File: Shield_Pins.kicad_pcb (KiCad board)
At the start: 2 copper layers, 76 x 38.3 mm, 19 parts, among them J1 Conn_01x04_Male, J2 Conn_01x06_Male, J3 Conn_01x06_Male, J4 Conn_01x04_Male, J5 Conn_01x01_Male, J6 Conn_01x06_Male, J7 Conn_01x15_Male, J8 Conn_01x15_Male, J9 Conn_01x02_Male, U1 ADXL343, U2 AZ1117

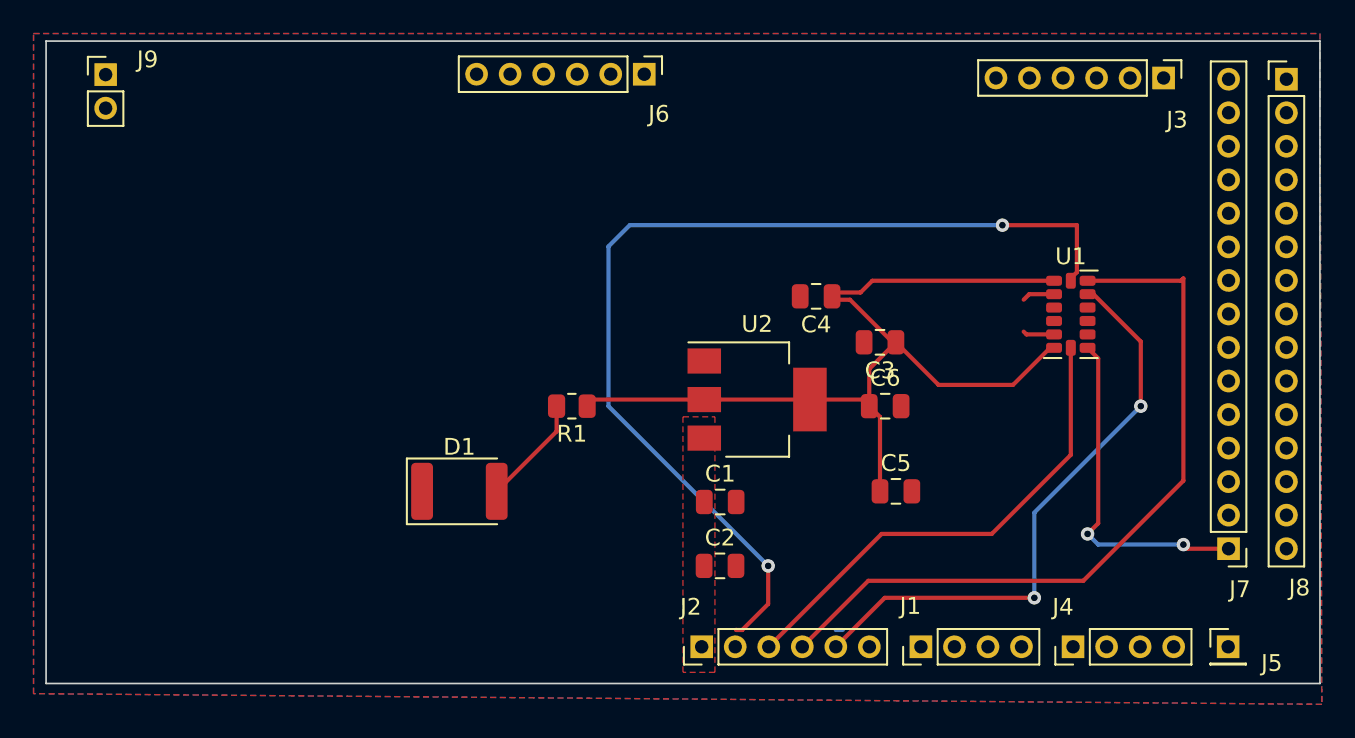
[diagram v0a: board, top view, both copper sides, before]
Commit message: Finished shield design
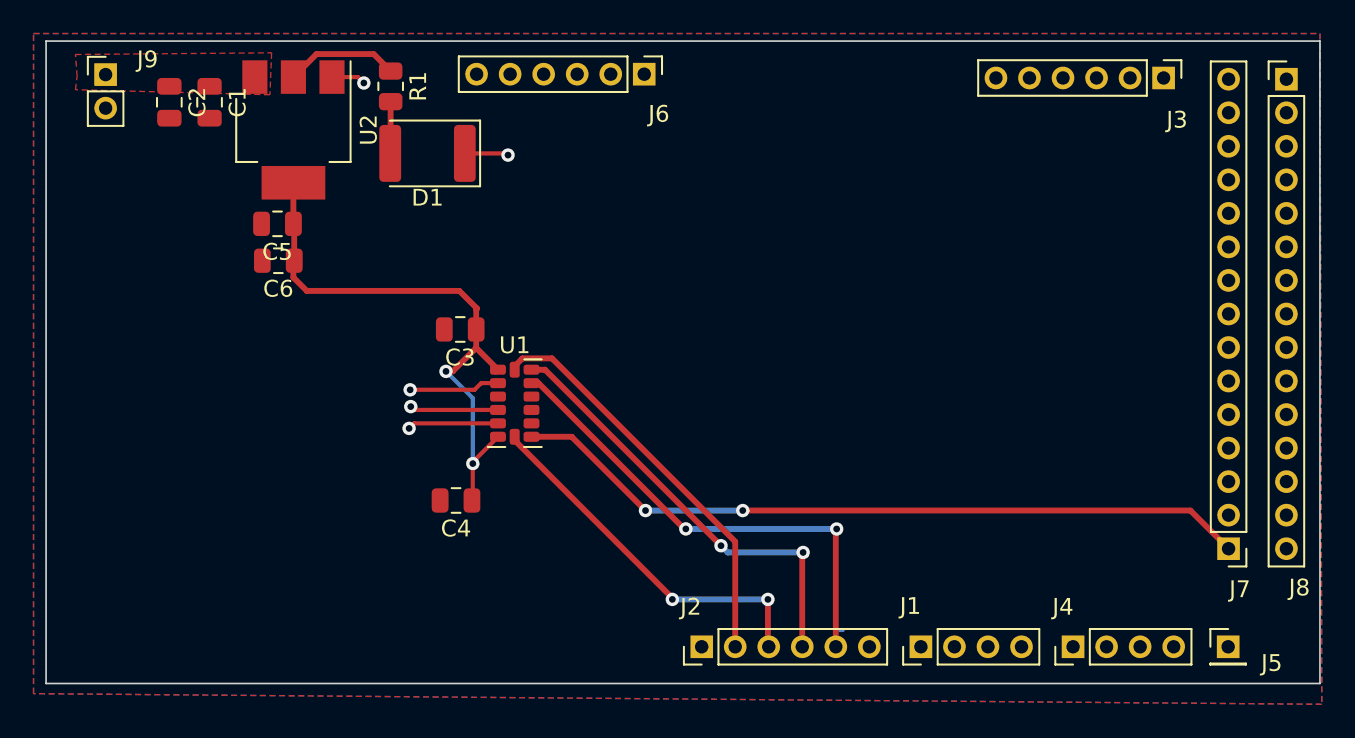
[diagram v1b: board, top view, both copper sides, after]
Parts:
- moved C2 42.9 mm to (97.0, 74.0), turned to -90 degrees
- moved C5 40.2 mm to (103.5, 81.2), turned to 180 degrees
- moved C1 38.7 mm to (99.4, 74.0), turned to -90 degrees
- moved C6 37.2 mm to (103.5, 83.4), turned to 180 degrees
- moved U1 33.6 mm to (117.6, 91.9)
- moved U2 32.0 mm to (104.4, 75.6), turned to -90 degrees
- moved C3 25.0 mm to (114.3, 87.5)
- moved C4 24.7 mm to (114.1, 97.7)
- moved R1 21.9 mm to (110.2, 73.0), turned to -90 degrees
- moved D1 20.2 mm to (112.4, 77.0), turned to 180 degrees
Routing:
- net IO.SCK: track 59.8 -> 24.4 mm, vias 2 -> 0
- net IO7: track 20.4 -> 44.4 mm
- net IO.SDI: track 44.7 -> 26.4 mm, vias 0 -> 2
- net GND: track 3.83 -> 20.8 mm, vias 0 -> 5
- net 3.3V: track 56.9 -> 41.8 mm, vias 0 -> 2
- net IO.CSB: track 29.1 -> 22.1 mm, vias 0 -> 2
- net IO.SDO: track 35.3 -> 28.8 mm
- net Net-(D1-Pad2): track 6.56 -> 3.10 mm
